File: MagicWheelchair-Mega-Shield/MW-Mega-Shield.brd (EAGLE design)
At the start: 87.3 x 58.4 mm, 20 parts

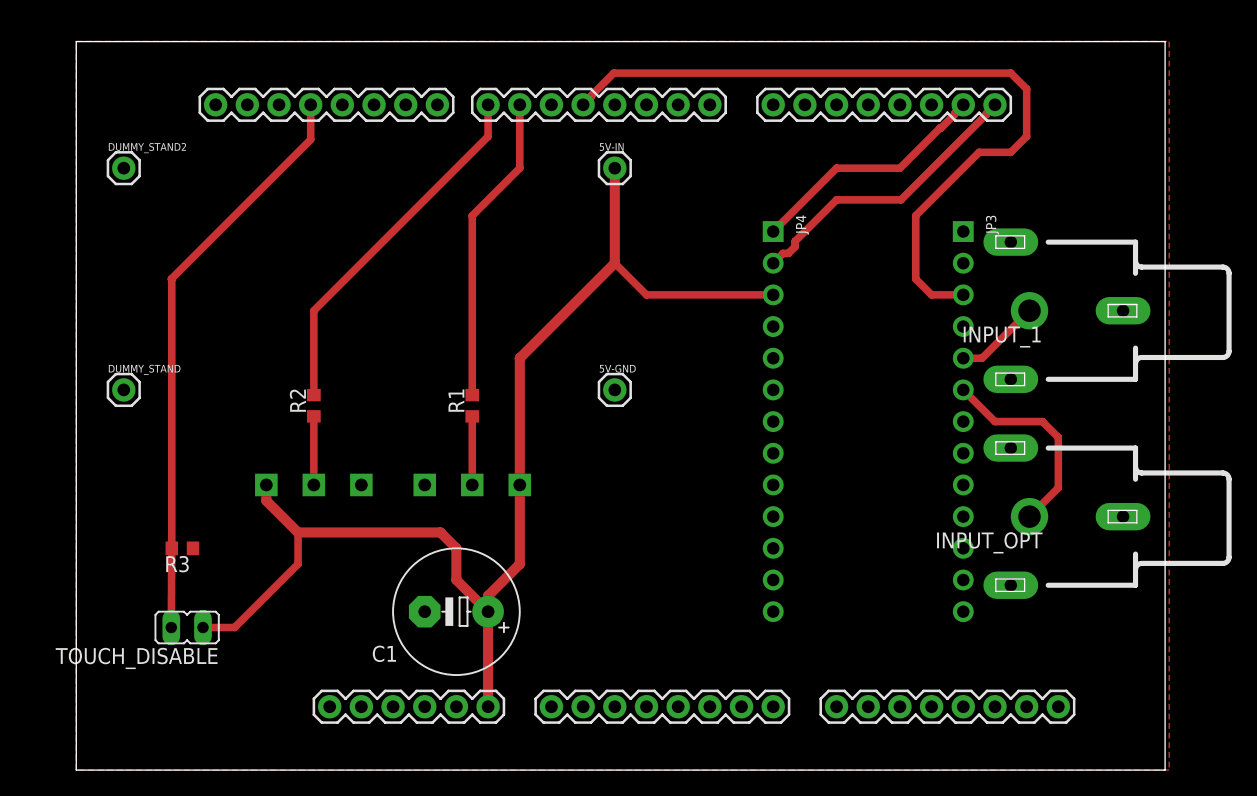
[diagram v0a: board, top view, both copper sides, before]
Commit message: Update PCB, better PNGs
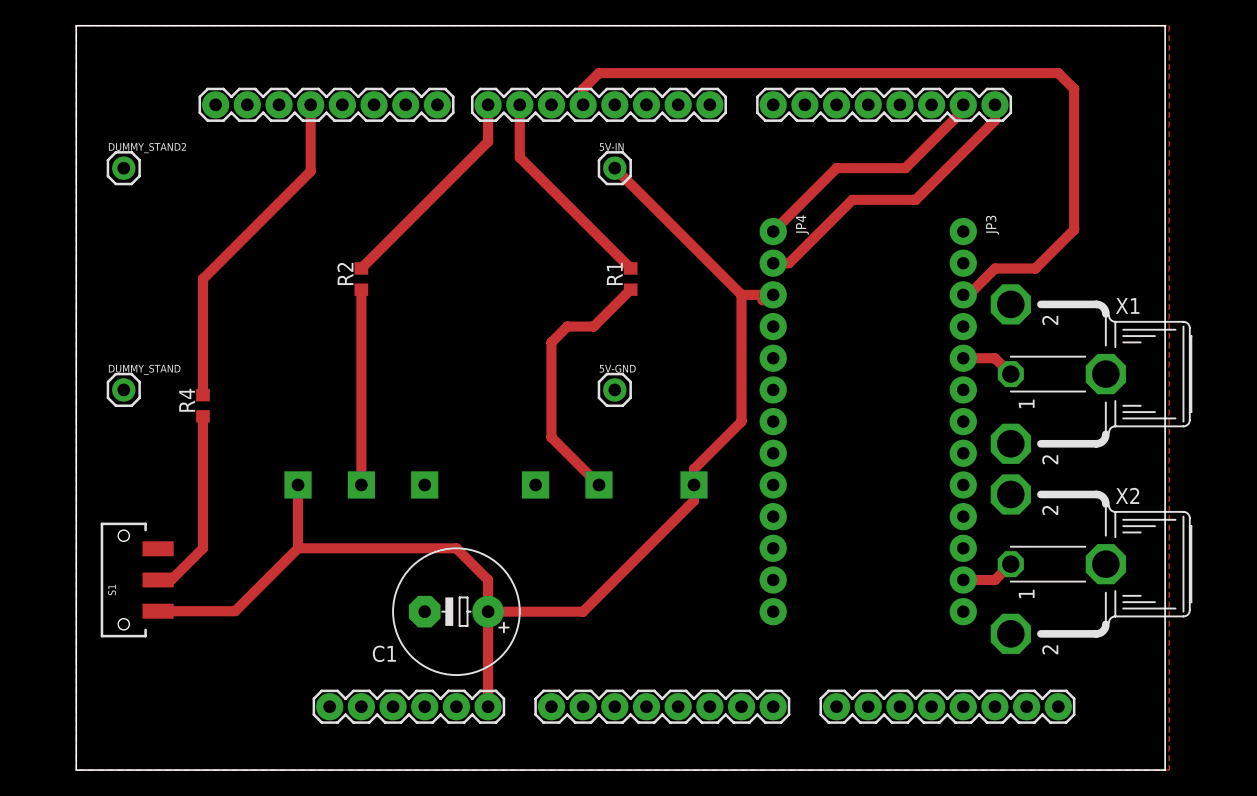
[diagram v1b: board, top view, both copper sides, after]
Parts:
- removed INPUT_1, INPUT_OPT: 736880-49, con-conrad:736880-49
- removed R3: 30kOhm, rcl:R0603
- removed TOUCH_DISABLE: (no value), jumper:JP1
- added R4: 30kOhm, rcl:R0603
- added S1: (no value), SparkFun-Retired:SWITCH_SPDT_SMD
- added X1, X2: TOBU3, con-hirschmann:TOBU3
- moved R1 16.3 mm to (52.1, 59.7)
- moved UNDER_VIN 14.0 mm to (57.1, 43.2)
- moved R2 10.9 mm to (30.5, 59.7)
- moved FIRE_DATA 10.2 mm to (49.5, 43.2)
- moved UNDER_GND 8.89 mm to (44.5, 43.2)
- moved FIRE_GND 5.08 mm to (35.6, 43.2)
- moved UNDER_DATA 3.81 mm to (30.5, 43.2)
- moved FIRE_VIN 2.54 mm to (25.4, 43.2)
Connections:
- removed net CS8: JP3.12
- new net CS2: JP3.6
- new net N$3: R4.1, S1.2
- net GND: now also S1.3, X1.2, X1.2@1, X1.2@2, X2.2, X2.2@1, X2.2@2; no longer R3.1
- net INPUT_1: now also X1.1; no longer INPUT_1.2
- net INPUT_OPT: now also JP3.12, X2.1; no longer INPUT_OPT.2, JP3.6
- net TOUCH_DISABLE: now also R4.2; no longer R3.2, TOUCH_DISABLE.2
- net VIN: now also S1.1; no longer TOUCH_DISABLE.1
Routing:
- net TOUCH_DISABLE: track 46.6 -> 26.9 mm
- net FIRE_DATA: track 5.50 -> 21.1 mm
- net N$3: track 0.00 -> 15.2 mm
- net INPUT_OPT: track 16.5 -> 4.34 mm
- net N$2: track 29.1 -> 17.3 mm
- net UNDER_DATA: track 5.50 -> 15.7 mm
- net N$1: track 24.9 -> 16.8 mm
- net VIN: track 97.6 -> 101.1 mm
- net INPUT_1: track 6.89 -> 4.34 mm
- net TOUCH_RESET: track 61.9 -> 64.0 mm
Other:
- board size 87.3 x 58.4 mm -> 87.3 x 59.7 mm
